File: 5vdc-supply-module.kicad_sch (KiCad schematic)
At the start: 17 parts

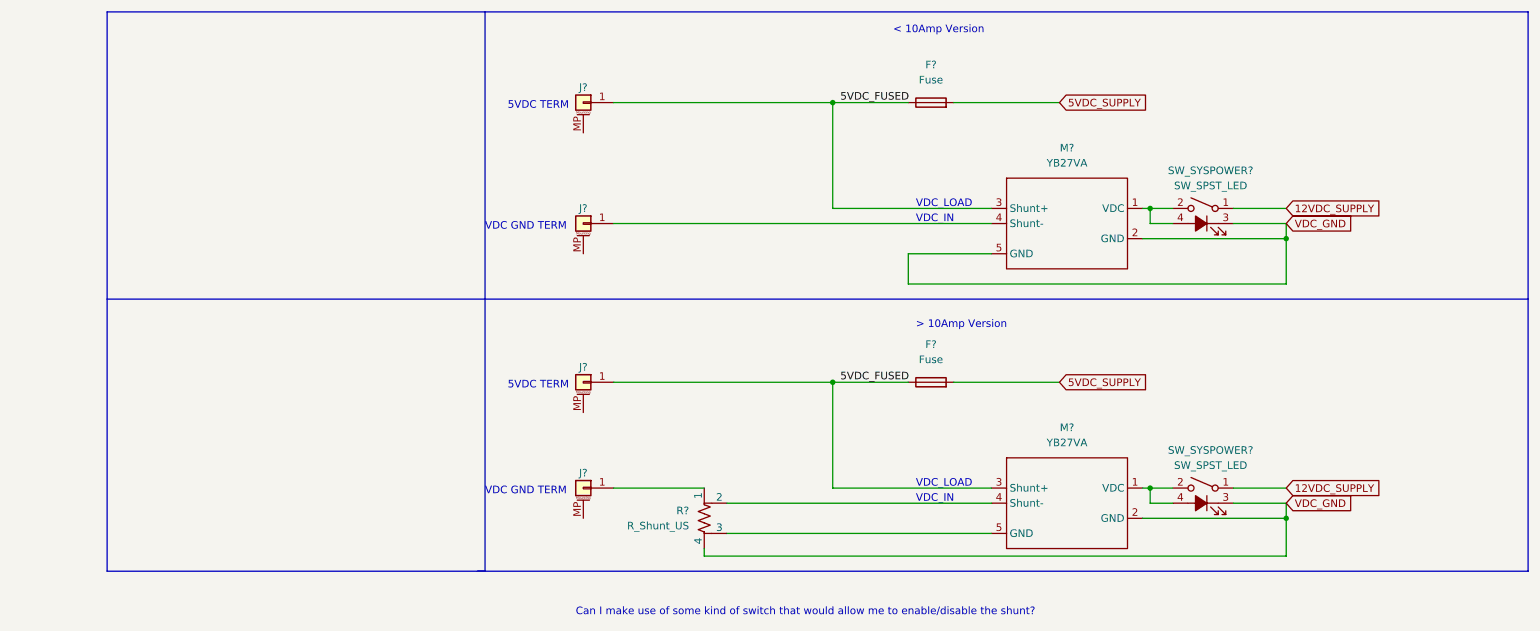
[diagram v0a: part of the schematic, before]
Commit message: Bunch more changes
Blah blah
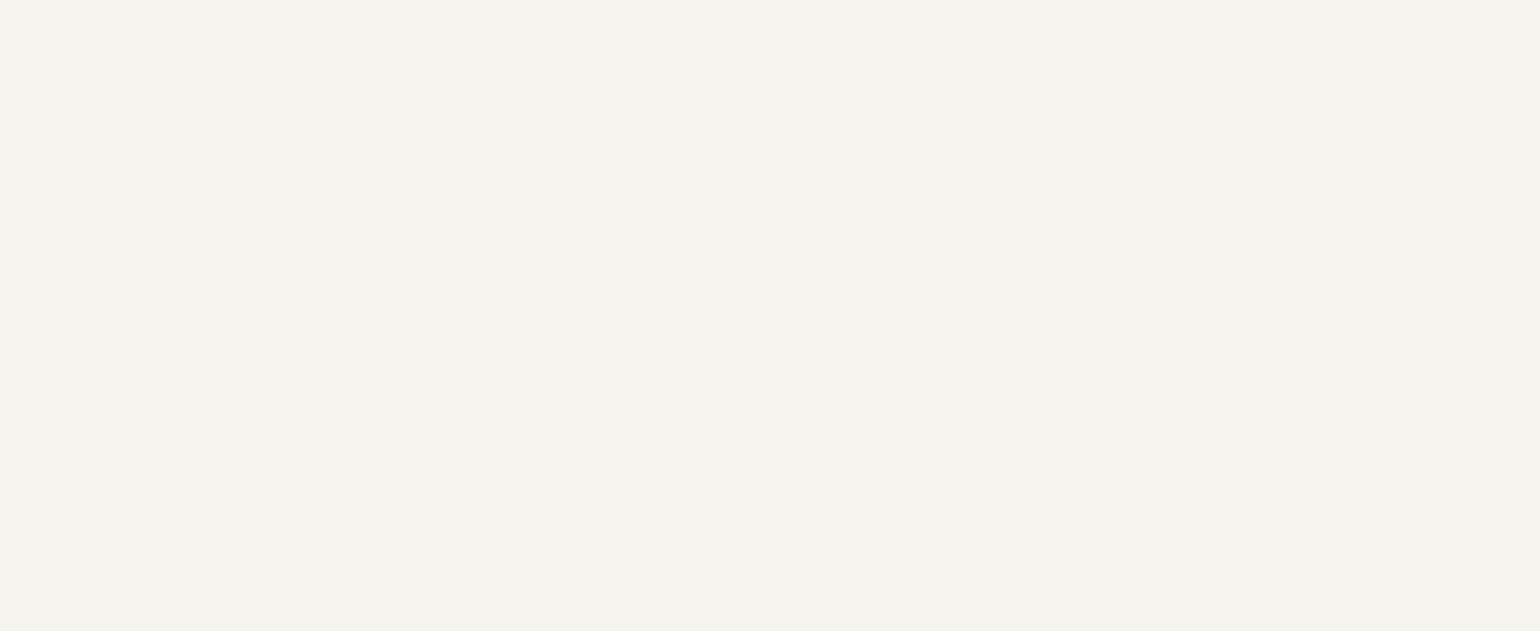
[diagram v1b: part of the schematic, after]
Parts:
- removed F? (x2): Fuse, symbol Device:Fuse
- removed J? (x4): Conn_01x01_MountingPin, symbol Connector_Generic_MountingPin:Conn_01x01_MountingPin
- removed M? (x2): YB27VA, symbol bvm-library:5_Pin_Meter_With_Ext_Shunt
- removed R?: R_Shunt_US, symbol Device:R_Shunt_US
- removed SW_SYSPOWER? (x2): SW_SPST_LED, symbol Switch:SW_SPST_LED
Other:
- note removed: "5VDC TERM"
- note removed: "< 10Amp Version"
- note removed: "> 10Amp Version"
- note removed: "Can I make use of some kind of switch that would allow me to enable/disable the shunt?"
- note removed: "VDC GND TERM"
- note removed: "VDC_IN"
- note removed: "VDC_LOAD"
- title: (none) -> Mr. Powers
